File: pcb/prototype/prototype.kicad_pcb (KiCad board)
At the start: 2 copper layers, 27.4 x 39 mm, 1 part

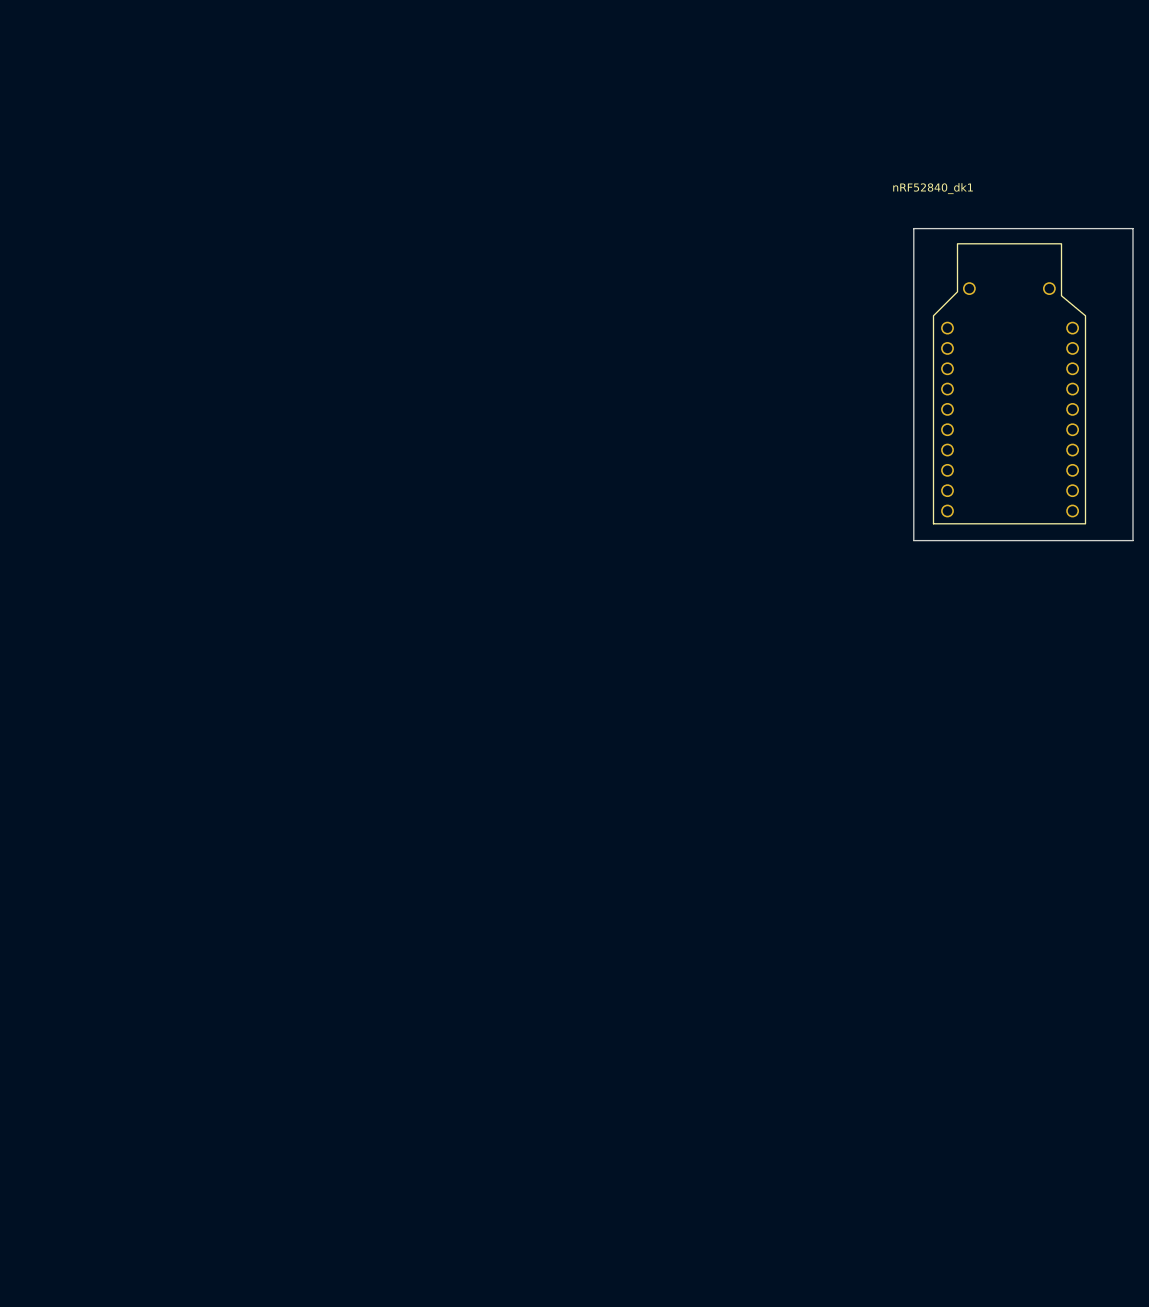
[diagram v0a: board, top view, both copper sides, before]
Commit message: v1 of prototype MO board
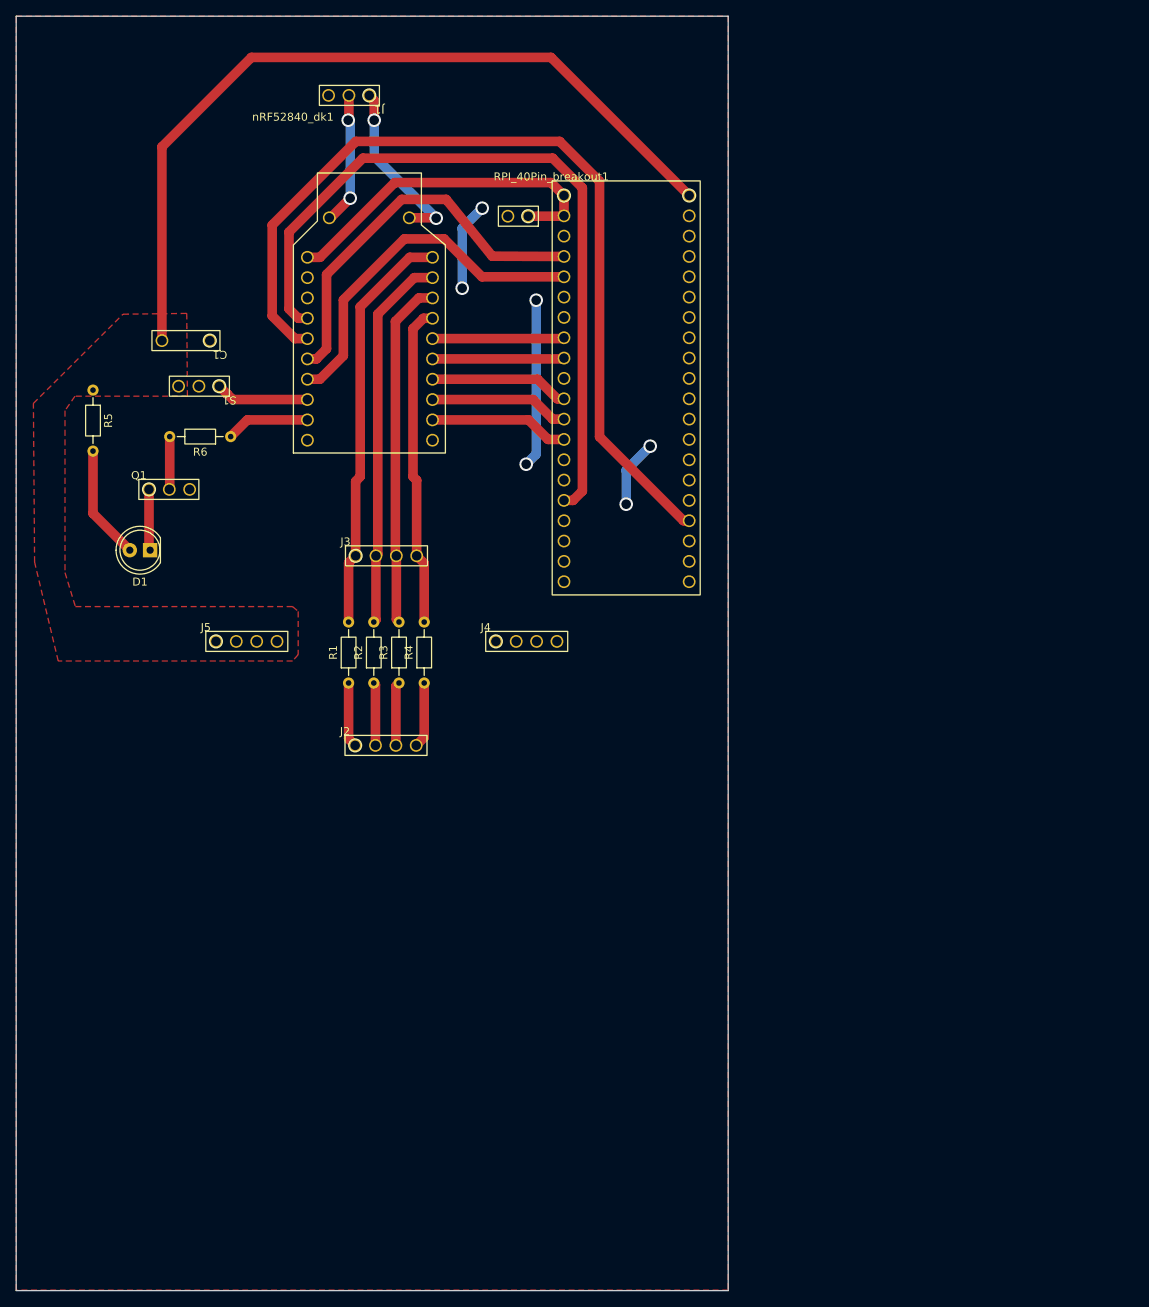
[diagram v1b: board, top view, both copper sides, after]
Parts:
- added C1: 1uF, prototypes:capacitor_generic, F.Cu at (45.5, 77.0)
- added D1: LED, LED_THT:LED_D5.0mm, F.Cu at (36.7, 102.0)
- added J1: SWD, prototypes:generic_3_pin, F.Cu at (65.4, 46.4)
- added J2: LOGIC_IN, prototypes:generic_4_pin, F.Cu at (61.1, 125.2)
- added J3: JMP_LOGIC, prototypes:generic_4_pin, F.Cu at (61.2, 101.5)
- added J4: JMP_GND, prototypes:generic_4_pin, F.Cu at (78.7, 112.2)
- added J5: JMP_3v3, prototypes:generic_4_pin, F.Cu at (43.7, 112.2)
- added J7: Display_power, prototypes:generic_2_pin, F.Cu at (85.3, 61.5)
- added Q1: 2N2222, prototypes:2N2222, F.Cu at (35.3, 93.2)
- added R1: 470R, Resistor_THT:R_Axial_DIN0204_L3.6mm_D1.6mm_P7.62mm_Horizontal, F.Cu at (61.5, 118.6)
- added R2: 470R, Resistor_THT:R_Axial_DIN0204_L3.6mm_D1.6mm_P7.62mm_Horizontal, F.Cu at (64.7, 118.6)
- added R3: 470R, Resistor_THT:R_Axial_DIN0204_L3.6mm_D1.6mm_P7.62mm_Horizontal, F.Cu at (67.8, 118.6)
- added R4: 470R, Resistor_THT:R_Axial_DIN0204_L3.6mm_D1.6mm_P7.62mm_Horizontal, F.Cu at (71.0, 118.6)
- added R5: 20R, Resistor_THT:R_Axial_DIN0204_L3.6mm_D1.6mm_P7.62mm_Horizontal, F.Cu at (29.6, 82.0)
- added R6: 220R, Resistor_THT:R_Axial_DIN0204_L3.6mm_D1.6mm_P7.62mm_Horizontal, F.Cu at (46.8, 87.8)
- added RPI_40Pin_breakout1: ~, prototypes:RPI_breakout_flipped, F.Cu at (86.9, 55.8)
- added S1: ~, prototypes:VS1838B, F.Cu at (46.6, 82.8)
- moved nRF52840_dk1 80.5 mm to (54.8, 54.8)
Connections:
- nRF52840_dk1 pad 1: unconnected-(nRF52840_dk1-SWDIO-Pad1) -> /DIO
- nRF52840_dk1 pad 10: unconnected-(nRF52840_dk1-0.09-Pad10) -> MOD2
- nRF52840_dk1 pad 11: unconnected-(nRF52840_dk1-0.10-Pad11) -> MOD3
- nRF52840_dk1 pad 12: unconnected-(nRF52840_dk1-1.10-Pad12) -> IR_TX
- nRF52840_dk1 pad 13: unconnected-(nRF52840_dk1-1.13-Pad13) -> IR_RX
- nRF52840_dk1 pad 14: unconnected-(nRF52840_dk1-1.15-Pad14) -> U0_TX
- nRF52840_dk1 pad 15: unconnected-(nRF52840_dk1-0.02-Pad15) -> U0_RX
- nRF52840_dk1 pad 16: unconnected-(nRF52840_dk1-0.29-Pad16) -> U1_RX
- nRF52840_dk1 pad 17: unconnected-(nRF52840_dk1-0.31-Pad17) -> U1_TX
- nRF52840_dk1 pad 18: unconnected-(nRF52840_dk1-GND-Pad18) -> GND
- nRF52840_dk1 pad 19: unconnected-(nRF52840_dk1-GND-Pad19) -> GND
- nRF52840_dk1 pad 2: unconnected-(nRF52840_dk1-SWDCLK-Pad2) -> /CLK
- nRF52840_dk1 pad 21: unconnected-(nRF52840_dk1-VBUS-Pad21) -> VBUS
- nRF52840_dk1 pad 22: unconnected-(nRF52840_dk1-VDD_OUT-Pad22) -> +1V35
- nRF52840_dk1 pad 3: unconnected-(nRF52840_dk1-0.13-Pad3) -> LOGIC0
- nRF52840_dk1 pad 4: unconnected-(nRF52840_dk1-0.15-Pad4) -> LOGIC1
- nRF52840_dk1 pad 5: unconnected-(nRF52840_dk1-0.17-Pad5) -> LOGIC2
- nRF52840_dk1 pad 6: unconnected-(nRF52840_dk1-0.20-Pad6) -> LOGIC3
- nRF52840_dk1 pad 7: unconnected-(nRF52840_dk1-0.22-Pad7) -> MOD0
- nRF52840_dk1 pad 8: unconnected-(nRF52840_dk1-0.24-Pad8) -> MOD1
- nRF52840_dk1 pad 9: unconnected-(nRF52840_dk1-1.00-Pad9) -> nRESET
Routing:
- net U1_RX: track 0.00 -> 111.7 mm
- net +3V3: track 0.00 -> 101.9 mm
- net U1_TX: track 0.00 -> 95.1 mm
- net LOGIC0: track 0.00 -> 51.6 mm
- net U0_RX: track 0.00 -> 49.2 mm
- net LOGIC1: track 0.00 -> 47.4 mm
- net U0_TX: track 0.00 -> 45.4 mm
- net VBUS: track 0.00 -> 43.6 mm
- net LOGIC2: track 0.00 -> 43.6 mm
- net GND: track 0.00 -> 40.5 mm, vias 0 -> 6
- net LOGIC3: track 0.00 -> 40.2 mm
- net /DIO: track 0.00 -> 22.2 mm, vias 0 -> 2
- net MOD3: track 0.00 -> 17.4 mm
- net nRESET: track 0.00 -> 17.4 mm
- net MOD2: track 0.00 -> 17.4 mm
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- added copper zone on F.Cu, net +3V3
- added copper zone on F.Cu, net GND
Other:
- board size 27.4 x 39 mm -> 89 x 159.3 mm
